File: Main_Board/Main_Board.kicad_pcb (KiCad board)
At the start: 4 copper layers, 80.5 x 75.6 mm, 68 parts, among them IC1 AZ1085CD-3.3TRG1, J1 PJ-037A, U1 STM32L152ZCTx, U2 LM386, Y1 ABM10W-16.0000MHZ-4-B1U-T3

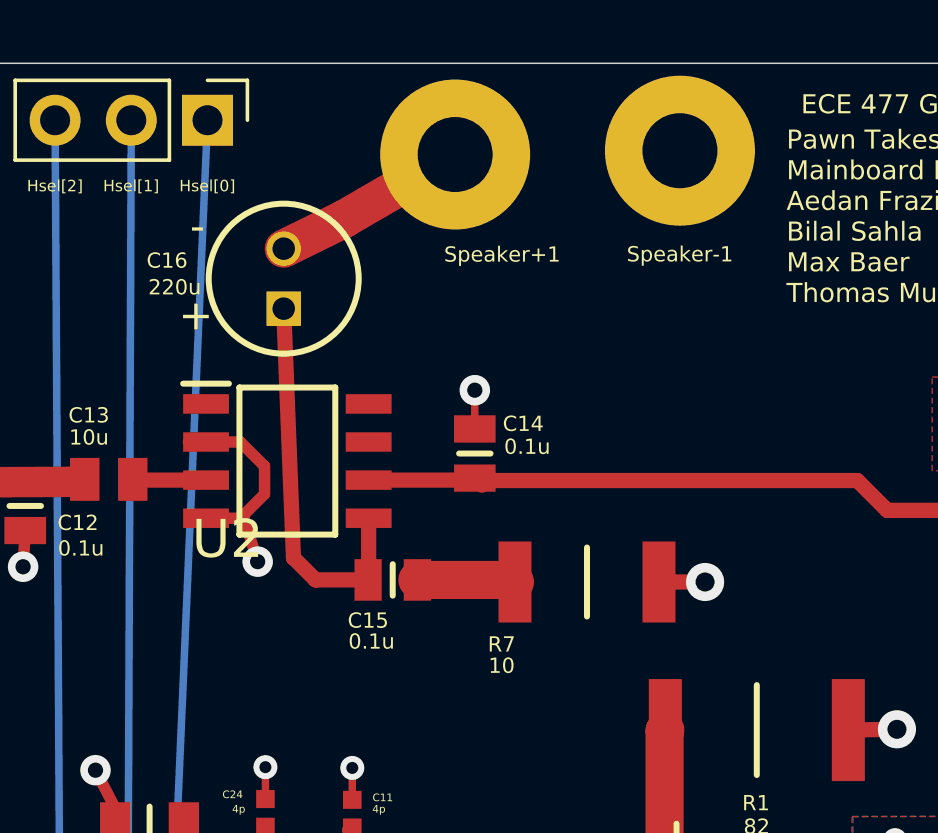
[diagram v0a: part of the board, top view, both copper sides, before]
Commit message: update
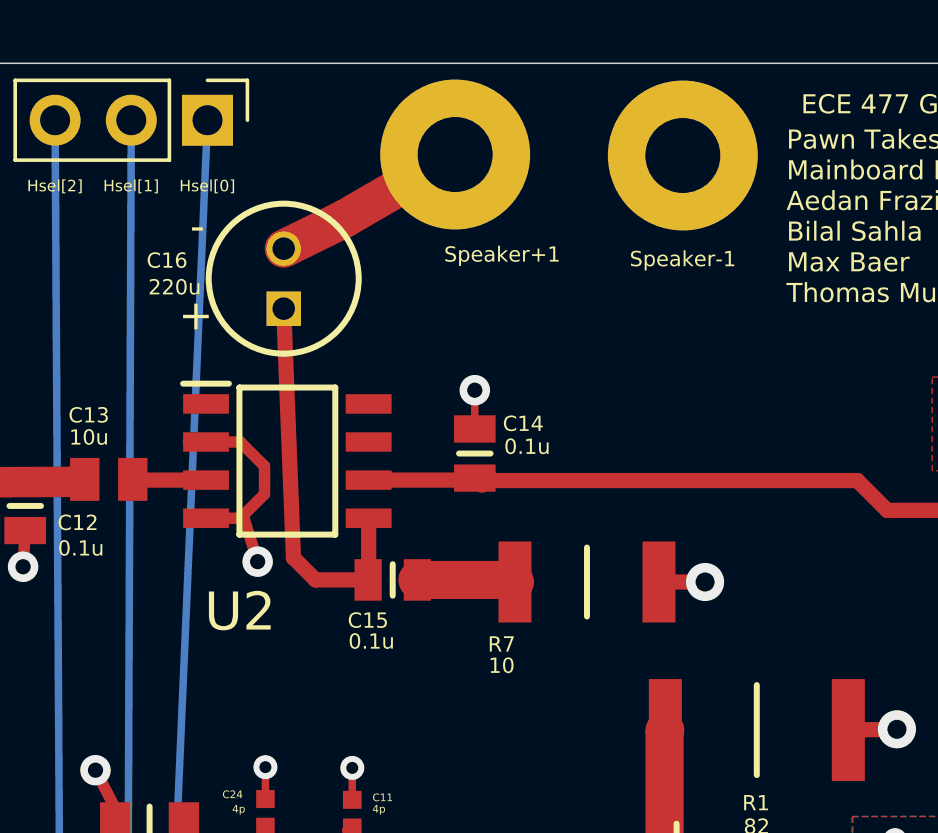
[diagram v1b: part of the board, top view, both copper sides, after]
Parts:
- moved Speaker-1 0.19 mm to (128.9, 27.9)
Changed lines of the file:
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@@
     (tags "Integrated Circuit")
     (attr smd)
-    (fp_text reference U2 (at -1.99136 2.60604) (layer F.SilkS)
-      (effects (font (size 1.27 1.27) (thickness 0.254)))
-    )
-    (fp_text value LM386 (at -2.0574 2.413) (layer F.SilkS) hide
+    (fp_text reference U2 (at -1.5748 5.0292) (layer F.SilkS)
+      (effects (font (size 1.27 1.27) (thickness 0.254)))
+    )
+    (fp_text value LM386 (at -1.4732 4.9784) (layer F.SilkS) hide
       (effects (font (size 1.27 1.27) (thickness 0.254)))
     )
@@
   )
   (module MountingHole:MountingHole_2.5mm_Pad (layer F.Cu)
-    (at 128.78308 27.75458)
+    (at 128.8796 27.9146)
     (descr "Mounting Hole 2.5mm")
     (tags "mounting hole 2.5mm")
@@
     (pad 3 smd rect (at 2.3 5.35 180) (size 1.5 2.5) (layers F.Cu F.Paste F.Mask)
       (net 17 +5V))
+    (model C:/Users/agf20/Downloads/ZLDO1117K33TC-pcb-part-libraries/SamacSys_Parts.3dshapes/IRLR8256PBF.stp
+      (offset (xyz -0 -1.524 0))
+      (scale (xyz 1 1 1))
+      (rotate (xyz 0 0 0))
+    )
   )
   (module Connector_PinHeader_2.54mm:PinHeader_1x09_P2.54mm_Vertical (layer F.Cu)
